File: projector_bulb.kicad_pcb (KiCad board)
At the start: 2 copper layers, 85.7 x 85.7 mm, 45 parts, among them J1 to_upright_+, J2 to_upright_-, J3 to_base, J4 Conn_02x02_Odd_Even, J5 Conn_02x02_Odd_Even, U1 PAM2863, U2 AP7381-33Y

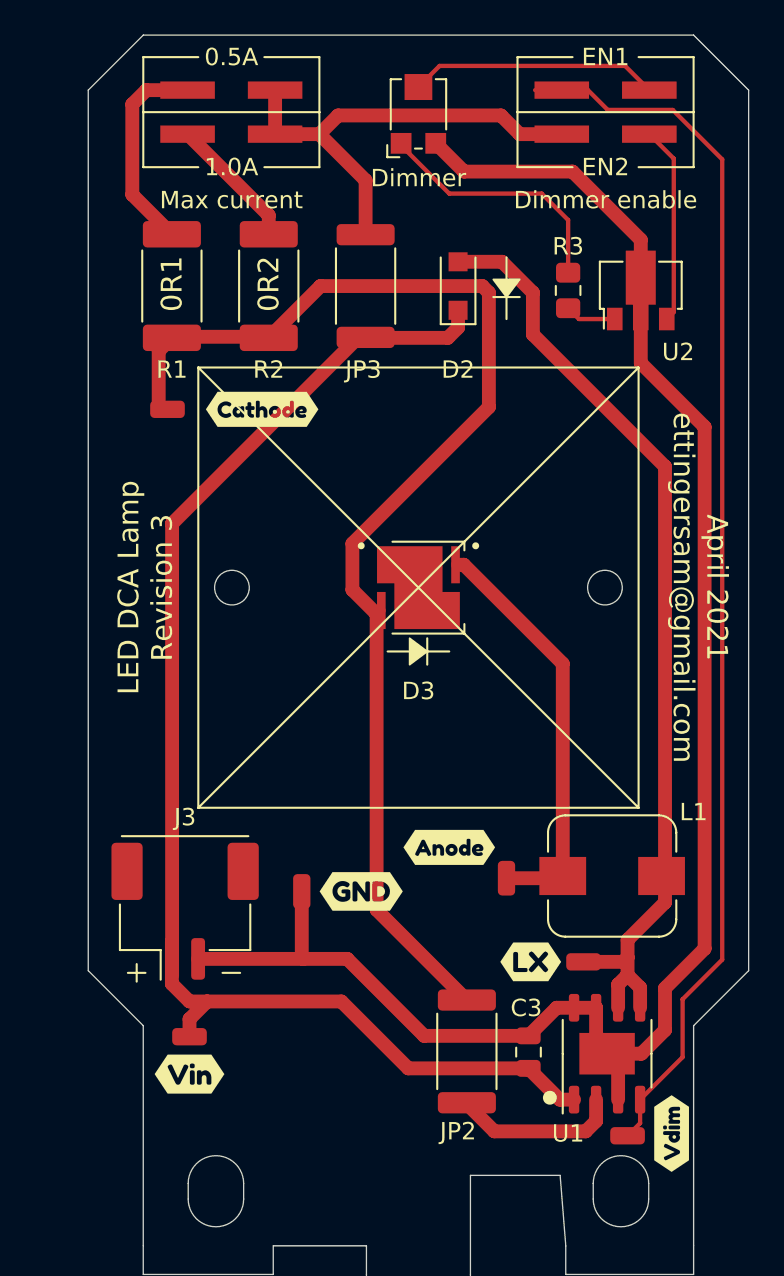
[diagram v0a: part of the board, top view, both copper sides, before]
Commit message: Routing optimizations
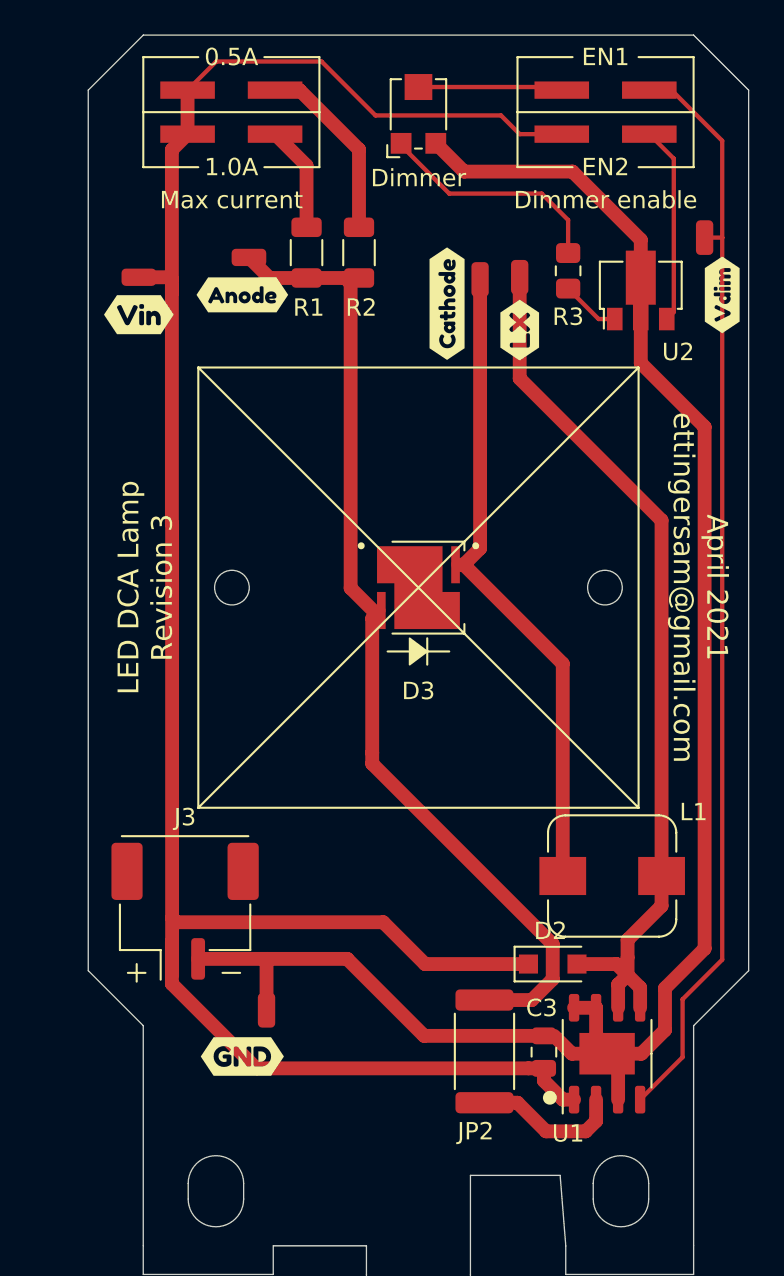
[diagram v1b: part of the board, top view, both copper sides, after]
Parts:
- removed JP3: Jumper_NC_Small, Resistor_SMD:R_2512_6332Metric
- D1: value D_Bridge_+-AA -> Bridge Rectifier
- D2: value D_Schottky -> Schottky
- D3: value LED_Small_ALT -> LED
- L1: value 47u -> 47μ
- R1: renamed from R2; footprint Resistor_SMD:R_2512_6332Metric_Pad1.52x3.35mm_HandSolder -> Resistor_SMD:R_1206_3216Metric
- R2: renamed from R1; footprint Resistor_SMD:R_2512_6332Metric_Pad1.52x3.35mm_HandSolder -> Resistor_SMD:R_1206_3216Metric
- moved TP4 52.0 mm to (143.5, 18.0), turned to 270 degrees
- moved svg2mod 48.5 mm to (144.5, 21.3)
- moved TP1 43.9 mm to (110.9, 20.3)
- moved svg2mod 43.9 mm to (110.9, 22.5)
- moved TP3 39.7 mm to (132.8, 20.3), turned to 90 degrees
- moved D2 39.5 mm to (134.7, 59.9), turned to 0 degrees
- moved svg2mod 36.5 mm to (132.8, 23.4), turned to 90 degrees
- moved TP6 34.6 mm to (130.6, 20.4)
- moved svg2mod 34.0 mm to (116.8, 21.3)
- moved svg2mod 12.3 mm to (128.7, 21.8), turned to 90 degrees
- moved svg2mod 11.7 mm to (116.8, 65.3)
- moved R2 11.0 mm to (123.6, 18.9)
- moved TP5 9.94 mm to (117.2, 19.2), turned to 180 degrees
- moved TP2 7.15 mm to (118.2, 62.6)
- moved R1 2.91 mm to (120.5, 18.9)
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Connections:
- J4 pad 1: Net-(J4-Pad1) -> VIN_UPRIGHT
- J4 pad 3: Net-(J4-Pad3) -> VIN_UPRIGHT
- J4 pad 4: Net-(J4-Pad2) -> Net-(J4-Pad4)
- J5 pad 3: Net-(J4-Pad2) -> VIN_UPRIGHT
- R1 pad 1: Net-(J4-Pad3) -> Net-(J4-Pad4)
- R2 pad 1: Net-(J4-Pad1) -> Net-(J4-Pad2)
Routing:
- net VIN_UPRIGHT: track 78.0 -> 127.5 mm
- net Net-(J4-Pad2): track 26.9 -> 10.7 mm
- net Net-(D3-Pad2): track 70.8 -> 56.2 mm
- net Net-(D3-Pad1): track 24.0 -> 37.7 mm
- net Net-(J4-Pad1): track 12.0 -> 0.00 mm
- net Net-(J4-Pad3): track 7.72 -> 0.00 mm
- net DIMMING: track 71.0 -> 63.7 mm
- net Net-(J5-Pad2): track 14.4 -> 8.09 mm
- net Net-(J4-Pad4): track 0.00 -> 6.12 mm
- net Net-(D2-Pad2): track 55.4 -> 51.9 mm
- net Net-(R3-Pad1): track 14.6 -> 13.4 mm
- net Net-(JP2-Pad1): track 9.59 -> 8.60 mm
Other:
- board text removed: "0R1"
- board text removed: "0R2"
